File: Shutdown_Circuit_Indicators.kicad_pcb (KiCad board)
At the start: 2 copper layers, 24.6 x 21 mm, 5 parts

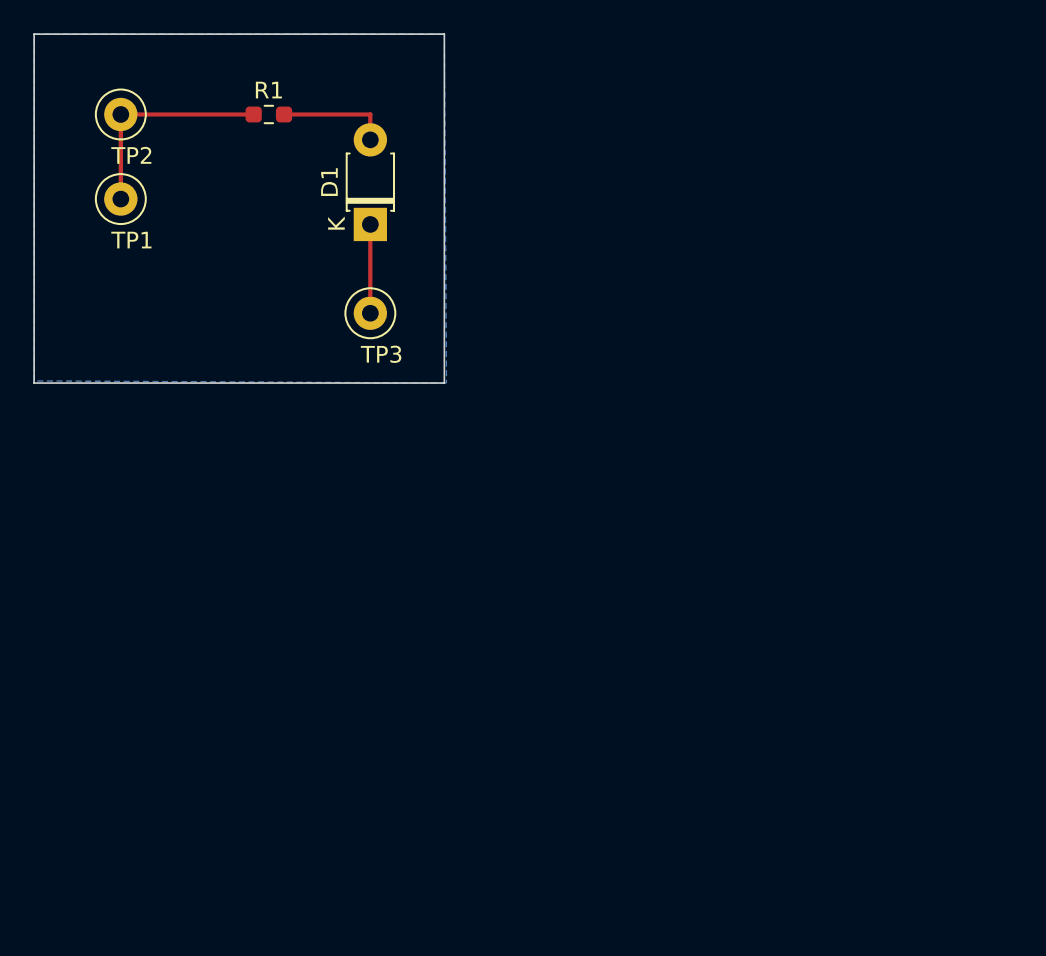
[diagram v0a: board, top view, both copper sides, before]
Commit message: Add files via upload
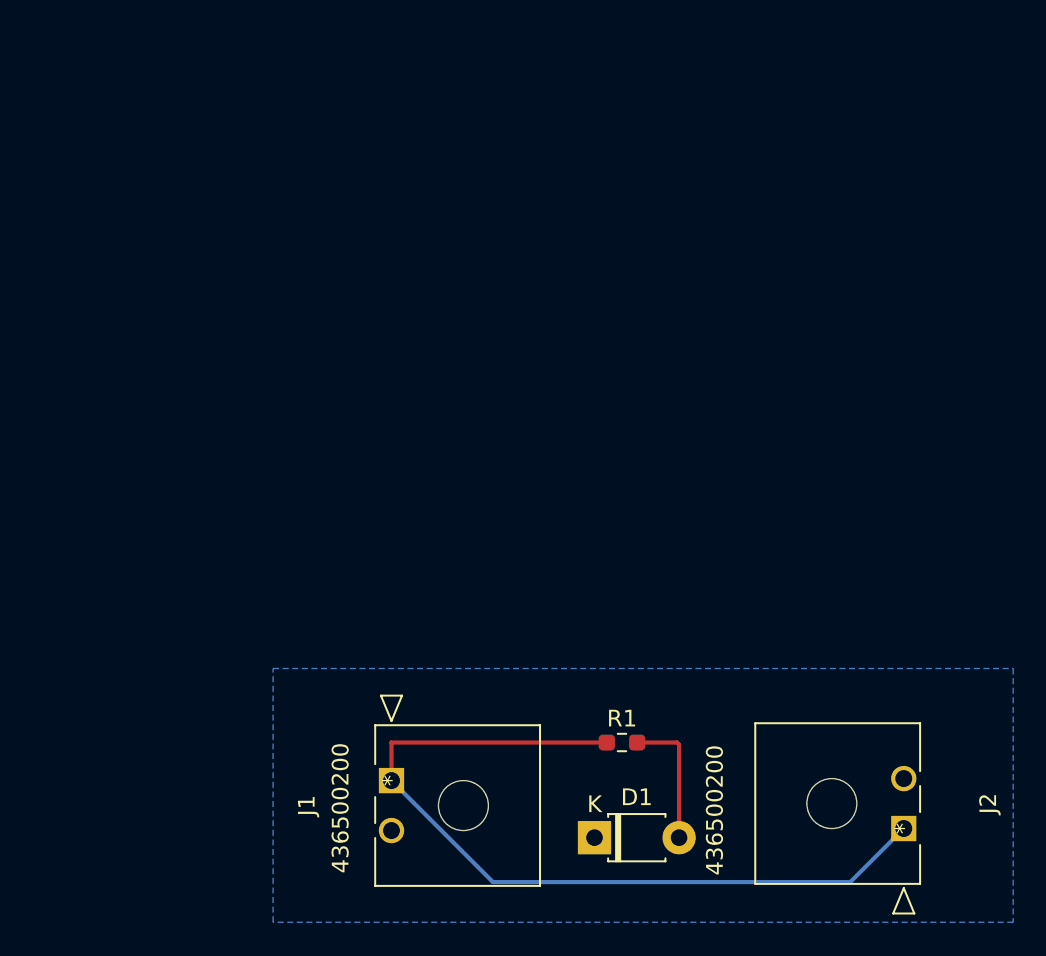
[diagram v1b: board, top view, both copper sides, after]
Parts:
- removed TP1: V_source-, TestPoint:TestPoint_Loop_D2.50mm_Drill1.0mm
- removed TP2: V_source+, TestPoint:TestPoint_Loop_D2.50mm_Drill1.0mm
- removed TP3: Ground, TestPoint:TestPoint_Loop_D2.50mm_Drill1.0mm
- added J1: 436500200, Global Libraries:436500200, F.Cu at (111.3, 82.9)
- added J2: 436500200, Global Libraries:436500200, F.Cu at (142.0, 85.8)
- R1: value 200 -> 1k
- moved R1 43.3 mm to (125.1, 80.6)
- moved D1 39.2 mm to (123.4, 86.4), turned to 0 degrees
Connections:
- R1 pad 1: V_source+ -> Input Power
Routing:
- net Input Power: track 0.00 -> 49.8 mm
- net V_source+: track 13.1 -> 0.00 mm
- net Ground: track 5.33 -> 0.00 mm
- net Net-(D1-Pad2): track 6.71 -> 8.16 mm
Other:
- board outline removed
